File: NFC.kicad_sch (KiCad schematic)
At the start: 36 parts, among them J1 Hirose, U2 PN5321A3HN_C1xx, Y1 27.12MHz

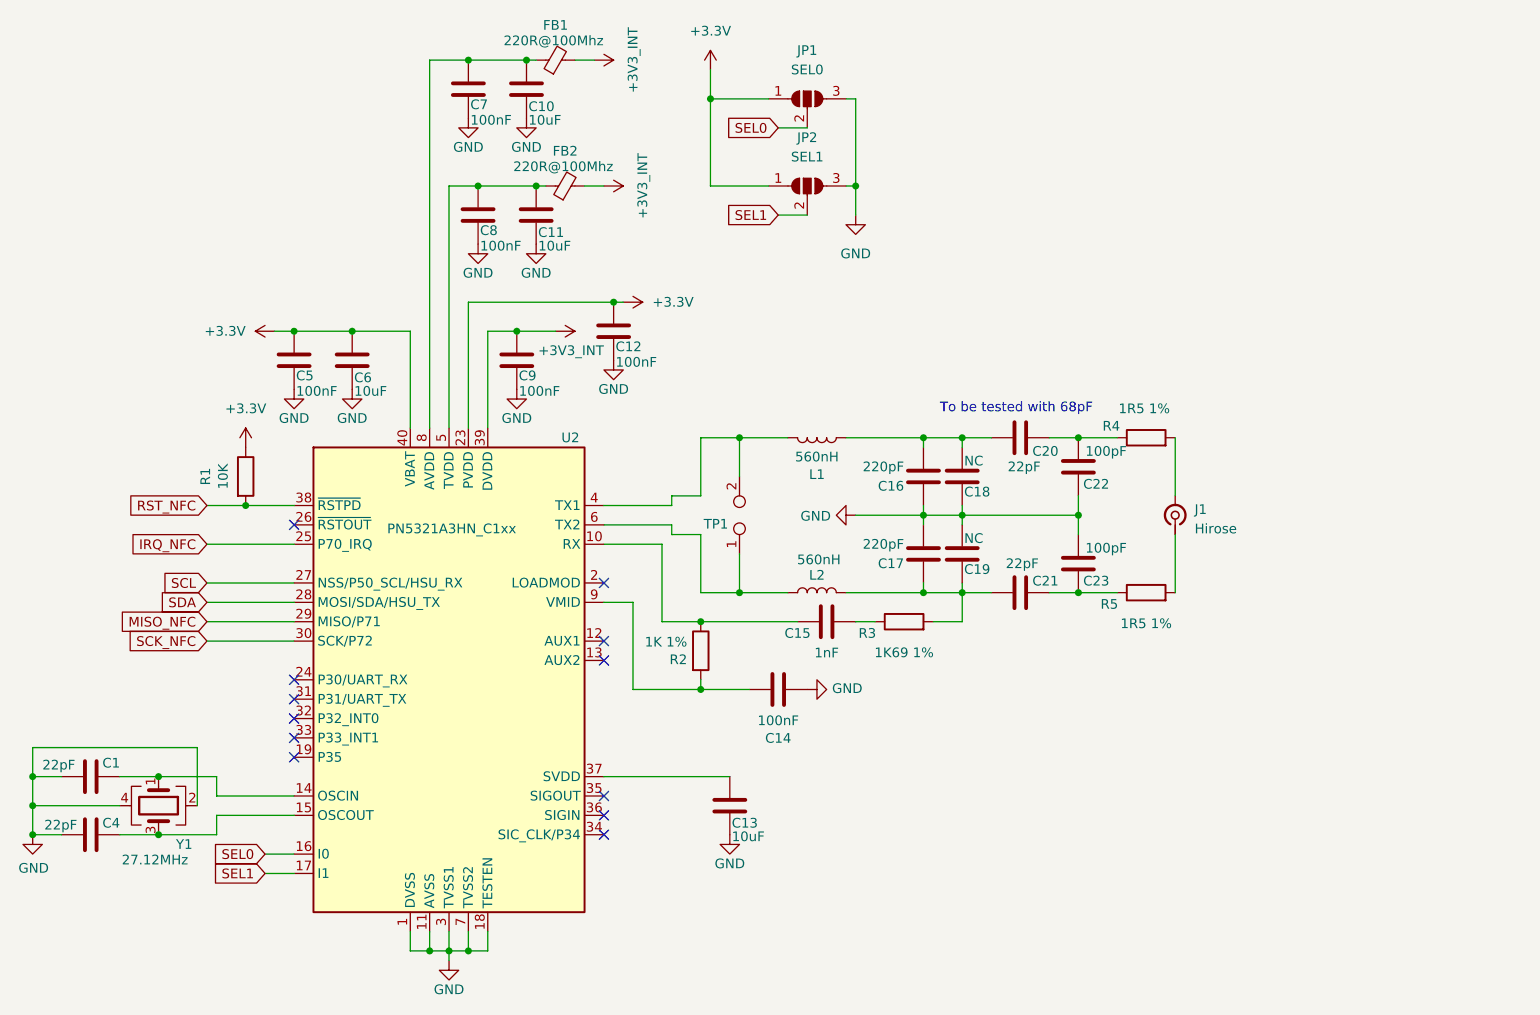
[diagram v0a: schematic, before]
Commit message: Start of layout
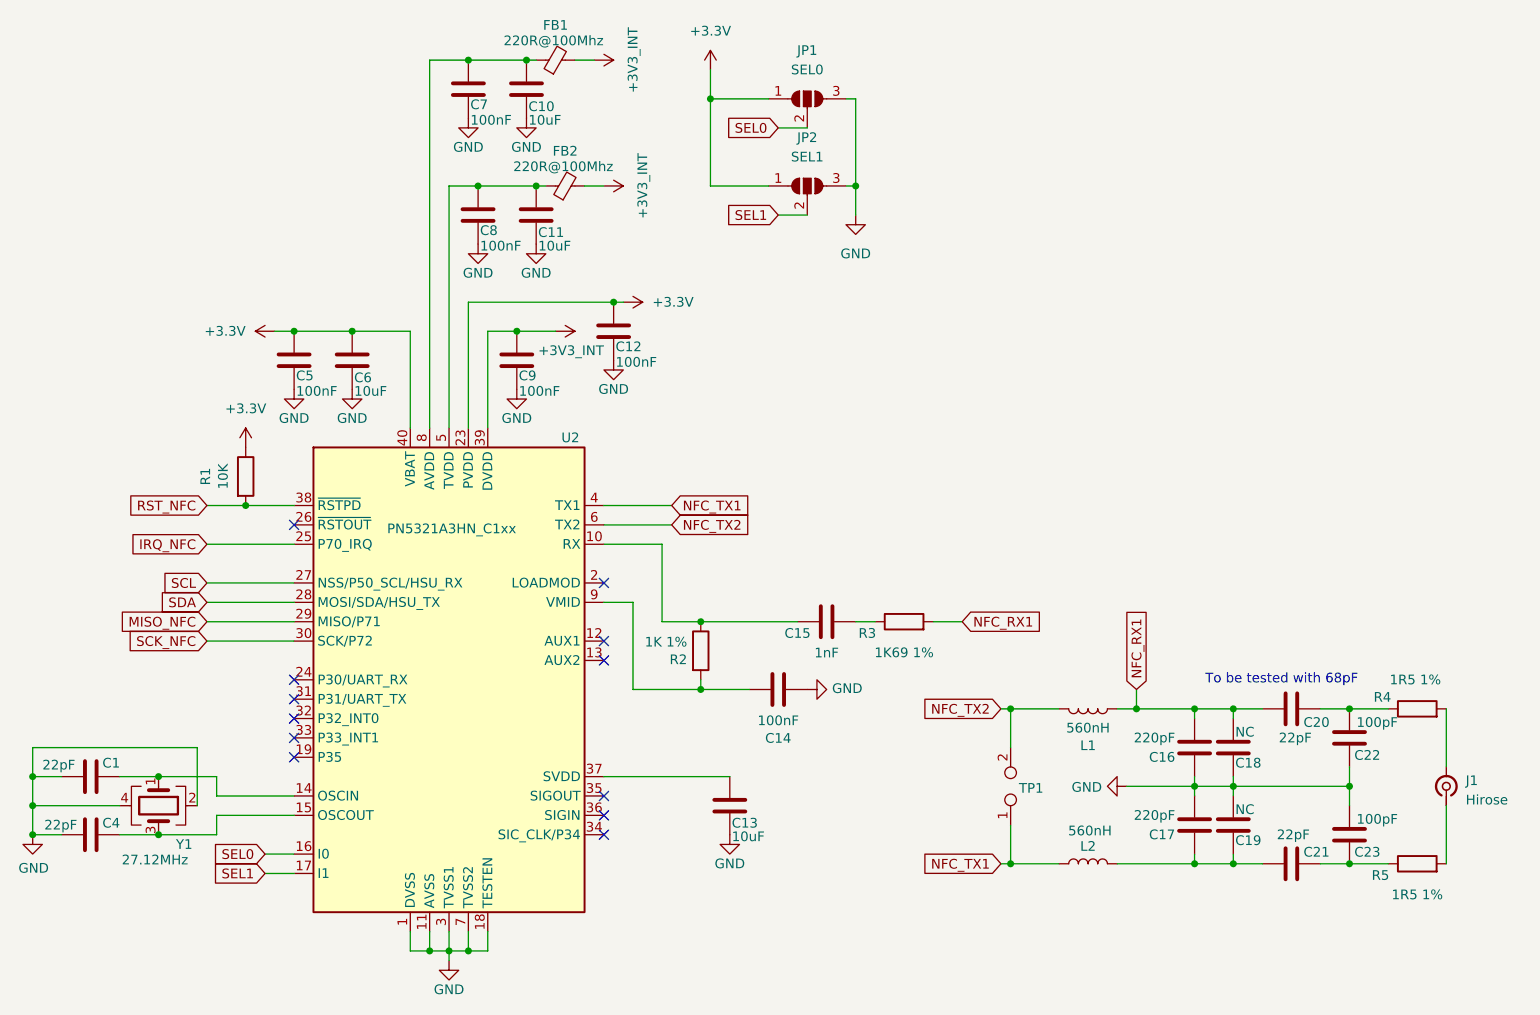
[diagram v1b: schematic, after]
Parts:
- C1, C14, C15, C16, C17, C20, C21, C23, C4: footprint RevK:C_0603 -> Capacitor_SMD_AKL:C_0603_1608Metric; symbol Device:C -> PCM_Capacitor_US_AKL:C_0603
- C18, C19, C5, C7, C8, C9: footprint Capacitor_SMD:C_0603_1608Metric -> Capacitor_SMD_AKL:C_0603_1608Metric; symbol Device:C -> PCM_Capacitor_US_AKL:C_0603
- C22: footprint RevK:C_0603 -> Capacitor_SMD:C_0603_1608Metric
- JP1, JP2: footprint (none) -> Jumper:SolderJumper-3_P2.0mm_Open_TrianglePad1.0x1.5mm
- L1, L2: footprint RevK:L_1206_1008 -> Inductor_SMD:L_0805_2012Metric
- R1, R2, R3, R4, R5: footprint RevK:R_0603 -> Resistor_SMD_AKL:R_0603_1608Metric; symbol Device:R -> PCM_Resistor_AKL:R_0603
- TP1: footprint RevK:PN532-RF-Test -> TestPoint:TestPoint_2Pads_Pitch2.54mm_Drill0.8mm
- Y1: footprint RevK:Crystal-3.2x2.5 -> Crystal:Crystal_SMD_3225-4Pin_3.2x2.5mm
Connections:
- net NFC_TX2: now reaches L1.2, TP1.2
- net NFC_TX2: now also U2.6 (TX2); no longer U2.4 (TX1)
- net NFC_TX1: now reaches L2.1, TP1.1
- net NFC_TX1: now also U2.4 (TX1); no longer U2.6 (TX2)
- net NFC_RX1: now reaches C16.2, C18.2, C20.1, L1.1
- net NFC_RX1: now also R3.2
- net at C17.2, C19.1, C21.1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: no longer R3.2
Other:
- moved on the sheet: C16, C17, C18, C19, C20, C21, C22, C23, J1, L1, L2, R4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
